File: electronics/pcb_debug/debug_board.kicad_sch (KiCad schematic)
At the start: 7 parts, among them J1 SWD Trace, J2 SWD Trace J Trace

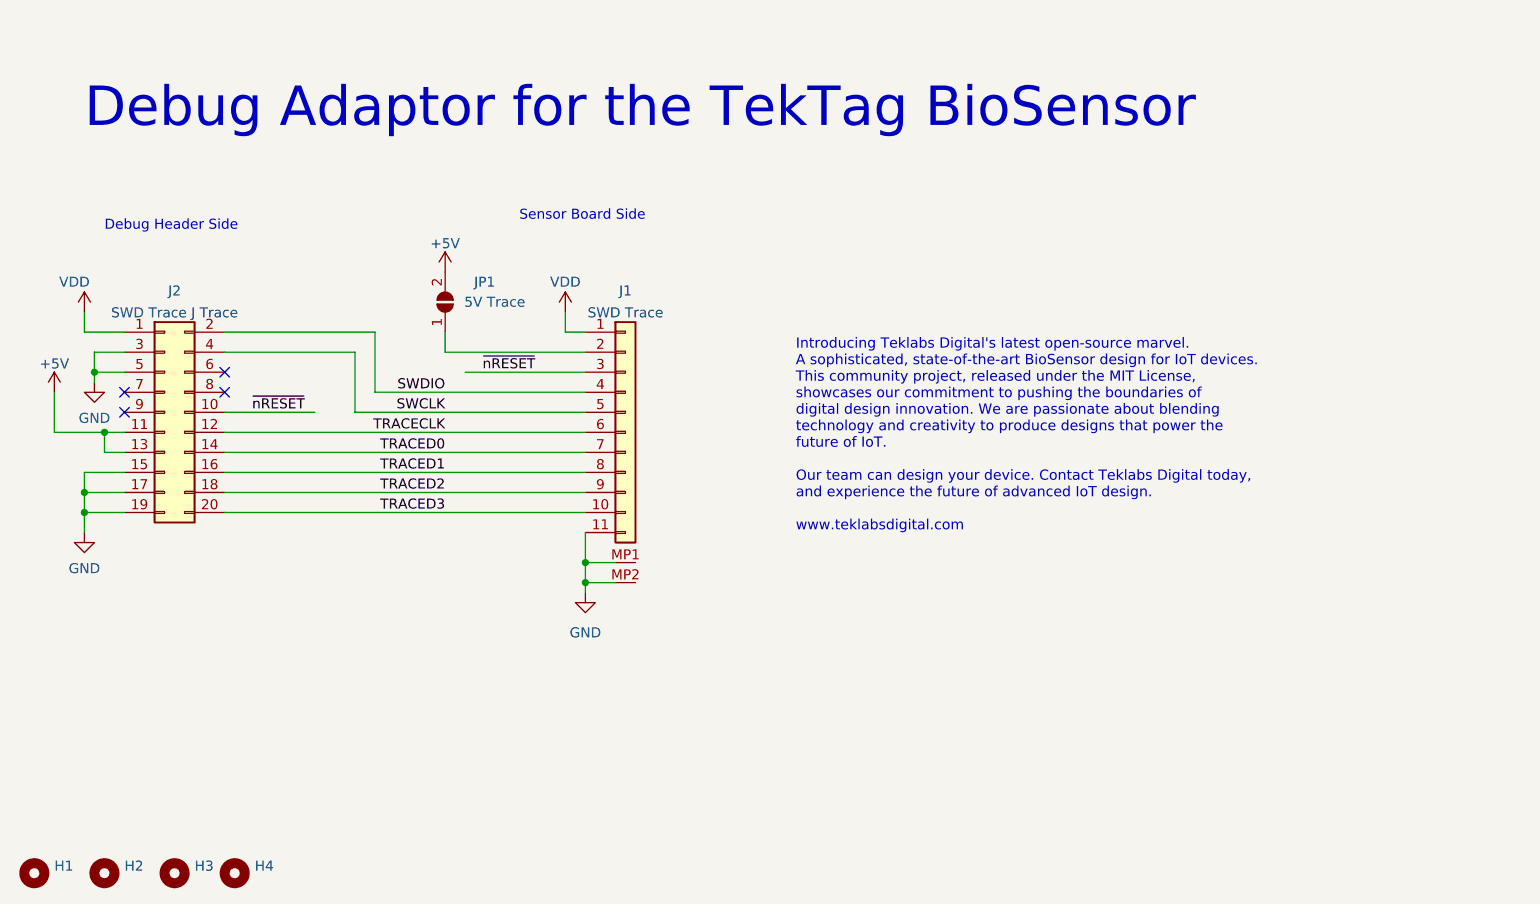
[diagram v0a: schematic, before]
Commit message: Hardware and Firmware udpates
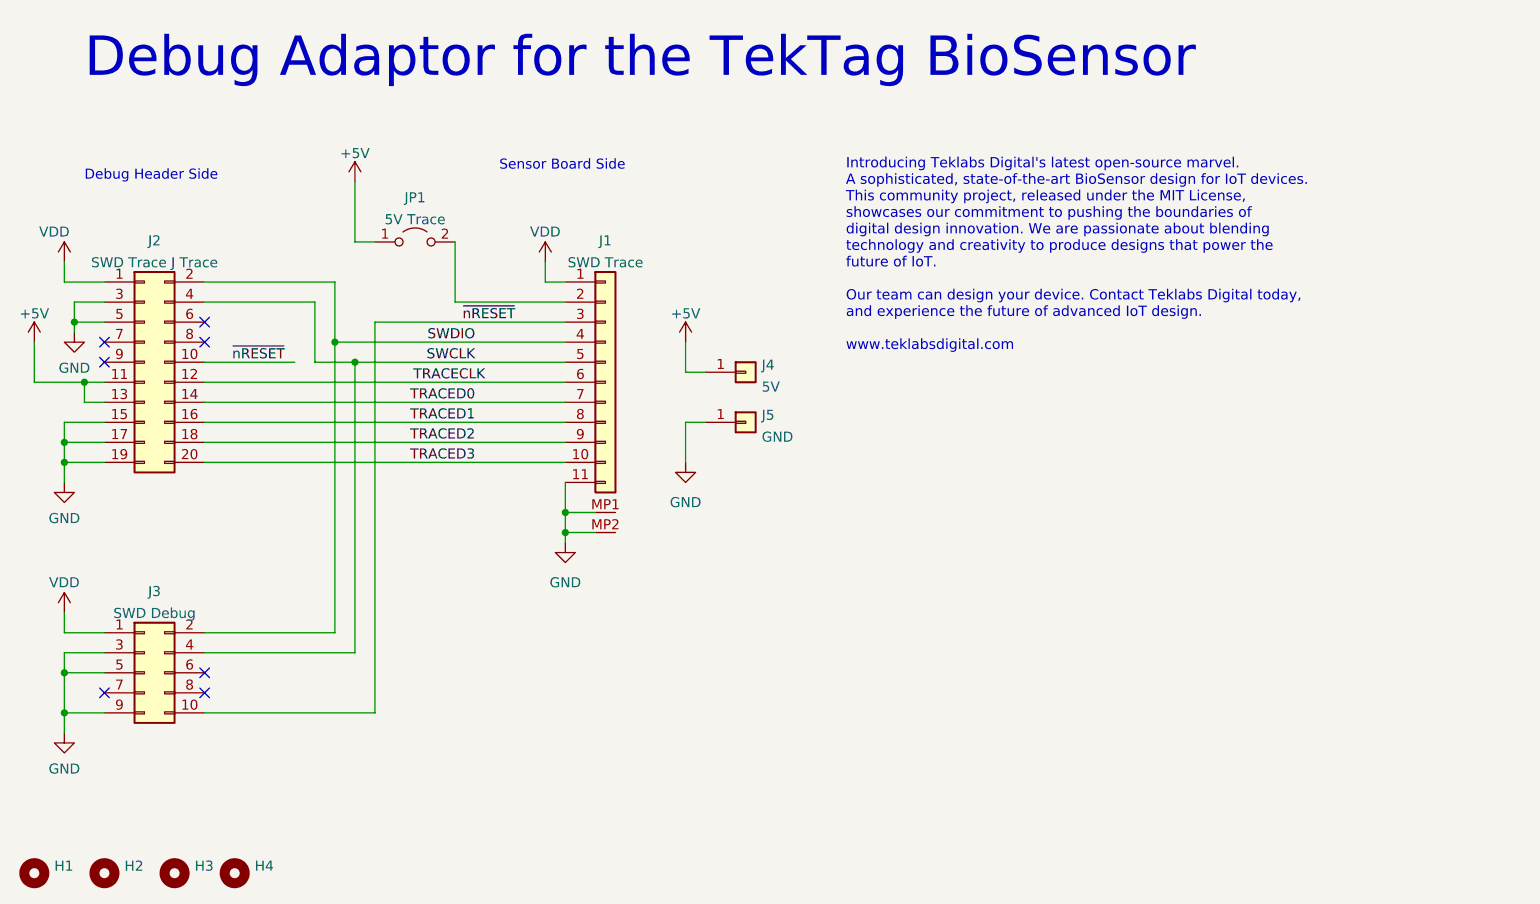
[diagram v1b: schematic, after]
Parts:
- removed JP1: 5V Trace, Jumper:SolderJumper-2_P1.3mm_Open_Pad1.0x1.5mm, symbol Jumper:SolderJumper_2_Open
- added J3: SWD Debug, Connector_PinHeader_1.27mm:PinHeader_2x05_P1.27mm_Vertical, symbol Connector_Generic:Conn_02x05_Odd_Even
- added J4: 5V, Connector_PinHeader_2.54mm:PinHeader_1x01_P2.54mm_Vertical, symbol Connector_Generic:Conn_01x01
- added J5: GND, Connector_PinHeader_2.54mm:PinHeader_1x01_P2.54mm_Vertical, symbol Connector_Generic:Conn_01x01
- added JP1: 5V Trace, Connector_PinHeader_2.54mm:PinHeader_1x02_P2.54mm_Vertical, symbol Jumper:Jumper_2_Open
- H1, H2, H3, H4: footprint MountingHole:MountingHole_2.5mm_Pad_Via -> MountingHole:MountingHole_3.7mm_Pad_TopBottom
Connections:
- net +5V: now also J4.1 (Pin_1), JP1.1 (A)
- net GND: now also J3.3 (Pin_3), J3.5 (Pin_5), J3.9 (Pin_9), J5.1 (Pin_1)
- net SWCLK: now also J3.4 (Pin_4)
- net SWDIO: now also J3.2 (Pin_2)
- net VDD: now also J3.1 (Pin_1)
- net ~{nRESET}: now also J3.10 (Pin_10)
- net at J1.2 (Pin_2): now also JP1.2 (B)
- no-connect marks 4 -> 7
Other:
- moved on the sheet: J1, J2
